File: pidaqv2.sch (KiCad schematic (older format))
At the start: 12 parts, among them J1 Raspberry_Pi_2_3, U1 INA2126E_250

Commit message: ads1261
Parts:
- removed C1, C8, C9: 0.1uF, Capacitor_SMD:C_0805_2012Metric_Pad1.15x1.40mm_HandSolder, symbol Device:C_Small
- removed J1: Raspberry_Pi_2_3, Connector_PinHeader_2.54mm:PinHeader_2x20_P2.54mm_Vertical, symbol Connector:Raspberry_Pi_2_3
- removed JAIN0: Screw_Terminal_01x10, TerminalBlock_TE-Connectivity:TerminalBlock_TE_1-282834-0_1x10_P2.54mm_Horizontal, symbol Connector:Screw_Terminal_01x10
- removed JAIN1: Screw_Terminal_01x12, TerminalBlock_TE-Connectivity:TerminalBlock_TE_1-282834-2_1x12_P2.54mm_Horizontal, symbol Connector:Screw_Terminal_01x12
- removed JLC1, JTC-1: Screw_Terminal_01x06, TerminalBlock_TE-Connectivity:TerminalBlock_TE_282834-6_1x06_P2.54mm_Horizontal, symbol Connector:Screw_Terminal_01x06
- removed MK1, MK2, MK3: MountingHole_Pad, MountingHole:MountingHole_2.7mm_M2.5_ISO14580_Pad, symbol Mechanical:MountingHole_Pad
- removed U1: INA2126E_250, footprints:INA2126E&slash_250, symbol ina2126:INA2126E_250
- added C101, C102: 0.1uF, Capacitor_SMD:C_0603_1608Metric, symbol Device:C
- added H101, H102, H103, H104: MountingHole, MountingHole:MountingHole_3.2mm_M3_ISO7380, symbol Mechanical:MountingHole
- added J101: Conn_02x04_Odd_Even, Connector_PinHeader_2.54mm:PinHeader_2x04_P2.54mm_Vertical, symbol Connector_Generic:Conn_02x04_Odd_Even
- added J102: Conn_01x03, Connector_PinHeader_2.54mm:PinHeader_1x03_P2.54mm_Vertical, symbol Connector_Generic:Conn_01x03
- added J103: Screw_Terminal_01x10, TerminalBlock_Phoenix:TerminalBlock_Phoenix_MKDS-1,5-10-5.08_1x10_P5.08mm_Horizontal, symbol Connector:Screw_Terminal_01x10
- added J104, J106: Screw_Terminal_01x08, TerminalBlock_Phoenix:TerminalBlock_Phoenix_MPT-0,5-8-2.54_1x08_P2.54mm_Horizontal, symbol Connector:Screw_Terminal_01x08
- added J105: Screw_Terminal_01x06, TerminalBlock_Phoenix:TerminalBlock_Phoenix_MKDS-3-6-5.08_1x06_P5.08mm_Horizontal, symbol Connector:Screw_Terminal_01x06
- added J107: Conn_01x01_Female, Connector_PinHeader_2.54mm:PinHeader_1x01_P2.54mm_Vertical, symbol Connector:Conn_01x01_Female
- added U101: INA2126E_250, footprints:INA2126E&slash_250, symbol ins2126:INA2126E_250
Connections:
- net labels added: 2.5V, GNDREF, GPIO, TC-, TC0, TC1, TC2, TC3, TC4, TC5, TC6, TC7, ~CS0, ~CS1
- net labels removed: +2.5V, GNDPWR, ~CE0, ~CE1
- wire segments 70 -> 42
- no-connect marks 4 -> 5
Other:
- note removed: "ID_SD and ID_SC PINS:\nThese pins are reserved for HAT ID EEPROM.\n\nAt boot time this I2C interface will be\ninterrogated to look for an EEPROM\nthat identifes the attached board and\nallows automagic setup of the GPIOs\n(and optionally, Linux drivers).\n\nDO NOT USE these pins for anything other\nthan attaching an I2C ID EEPROM. Leave\nunconnected if ID EEPROM not required."
- note removed: "INA2126 comes with free 5x gain\n"
- note removed: "This ADC is set up for use of the internal PGA (GAINS).\nAll inputs should be in the range of 2.5V +/- 2V\n\nExcel calculator: https://www.ti.com/tool/ADS124S08-EXCEL-CALC-TOOL\n"
- note removed: "Tie negative inputs of thermocouples to +2.5V\n"

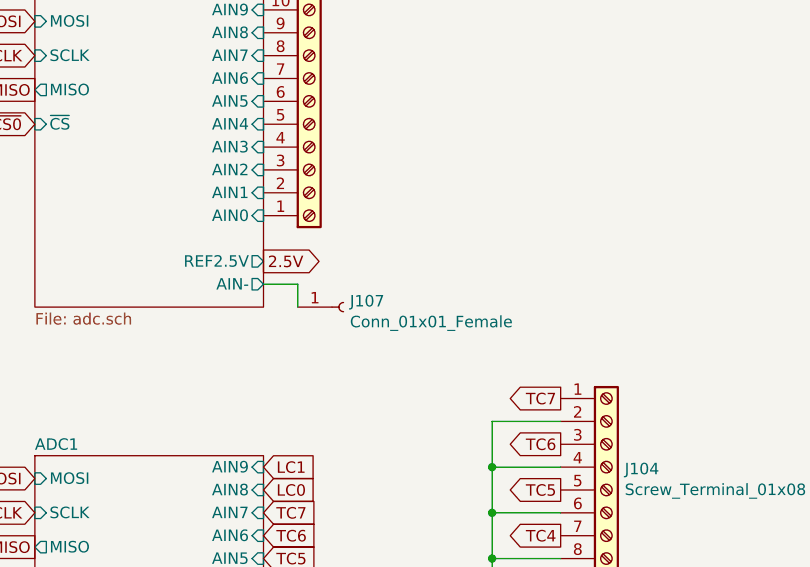
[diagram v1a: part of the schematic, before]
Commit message: last highfreq
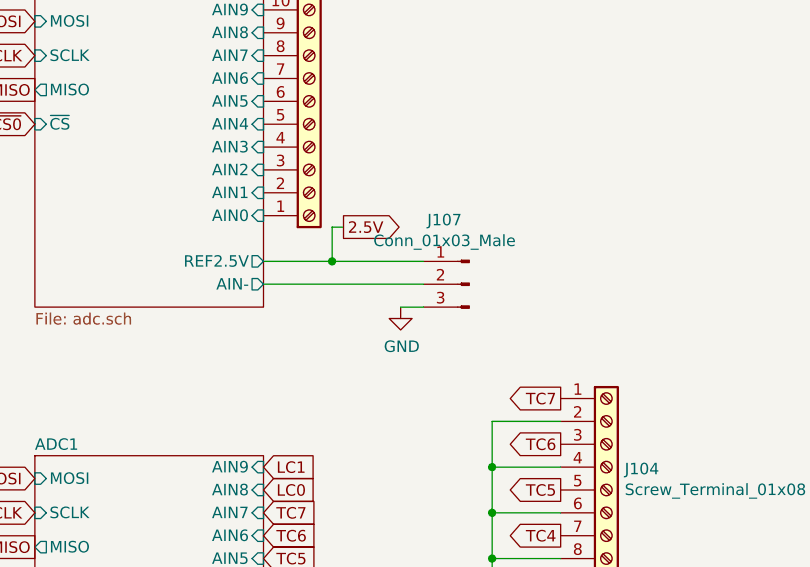
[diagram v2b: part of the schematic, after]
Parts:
- removed J107: Conn_01x01_Female, Connector_PinHeader_2.54mm:PinHeader_1x01_P2.54mm_Vertical, symbol Connector:Conn_01x01_Female
- added J107: Conn_01x03_Male, Connector_PinSocket_2.54mm:PinSocket_1x03_P2.54mm_Vertical, symbol Connector:Conn_01x03_Male
- J101, J102, J103, J104, J105, J106: DNP? (none) -> DNP
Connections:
- net 2.5V: now also J107.1 (Pin_1)
- net ADC0/AIN-: now also J107.2 (Pin_2)
- net GND: now also J107.3 (Pin_3)
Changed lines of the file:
@@
 F 2 "Connector_PinHeader_2.54mm:PinHeader_2x04_P2.54mm_Vertical" H 1400 1950 50  0001 C CNN
 F 3 "~" H 1400 1950 50  0001 C CNN
+F 4 "DNP" H 1400 1950 50  0001 C CNN "DNP?"
 	1    1400 1950
 	-1   0    0    -1
@@
 F 2 "TerminalBlock_Phoenix:TerminalBlock_Phoenix_MKDS-1,5-10-5.08_1x10_P5.08mm_Horizontal" H 2100 4050 50  0001 C CNN
 F 3 "~" H 2100 4050 50  0001 C CNN
+F 4 "DNP" H 2100 4050 50  0001 C CNN "DNP?"
 	1    2100 4050
 	1    0    0    1
@@
 F 2 "TerminalBlock_Phoenix:TerminalBlock_Phoenix_MKDS-3-6-5.08_1x06_P5.08mm_Horizontal" H 8350 5450 50  0001 C CNN
 F 3 "~" H 8350 5450 50  0001 C CNN
+F 4 "DNP" H 8350 5450 50  0001 C CNN "DNP?"
 	1    8350 5450
 	1    0    0    -1
@@
 	1    0    0    -1
 $EndComp
-Text GLabel 1900 4650 2    50   Output ~ 0
+Text GLabel 2250 4500 2    50   Output ~ 0
 2.5V
 Text GLabel 1900 6750 2    50   Output ~ 0
@@
 F 2 "TerminalBlock_Phoenix:TerminalBlock_Phoenix_MPT-0,5-8-2.54_1x08_P2.54mm_Horizontal" H 3400 5550 50  0001 C CNN
 F 3 "~" H 3400 5550 50  0001 C CNN
+F 4 "DNP" H 3400 5550 50  0001 C CNN "DNP?"
 	1    3400 5550
 	1    0    0    -1
@@
 F 2 "TerminalBlock_Phoenix:TerminalBlock_Phoenix_MPT-0,5-8-2.54_1x08_P2.54mm_Horizontal" H 3400 6550 50  0001 C CNN
 F 3 "~" H 3400 6550 50  0001 C CNN
+F 4 "DNP" H 3400 6550 50  0001 C CNN "DNP?"
 	1    3400 6550
 	1    0    0    -1
@@
 F 2 "Connector_PinHeader_2.54mm:PinHeader_1x03_P2.54mm_Vertical" H 1450 1200 50  0001 C CNN
 F 3 "~" H 1450 1200 50  0001 C CNN
+F 4 "DNP" H 1450 1200 50  0001 C CNN "DNP?"
 	1    1450 1200
 	1    0    0    -1
@@
 $EndComp
 $Comp
-L Connector:Conn_01x01_Female J107
-U 1 1 5F4B9AB1
-P 2250 4850
-F 0 "J107" H 2278 4876 50  0000 L CNN
-F 1 "Conn_01x01_Female" H 2278 4785 50  0000 L CNN
-F 2 "Connector_PinHeader_2.54mm:PinHeader_1x01_P2.54mm_Vertical" H 2250 4850 50  0001 C CNN
-F 3 "~" H 2250 4850 50  0001 C CNN
-	1    2250 4850
-	1    0    0    -1
-$EndComp
-Wire Wire Line
-	1900 4750 2050 4750
-Wire Wire Line
-	2050 4750 2050 4850
+L Connector:Conn_01x03_Male J107
+U 1 1 5F5328B6
+P 2800 4750
+F 0 "J107" H 2908 5031 50  0000 C CNN
+F 1 "Conn_01x03_Male" H 2908 4940 50  0000 C CNN
+F 2 "Connector_PinSocket_2.54mm:PinSocket_1x03_P2.54mm_Vertical" H 2800 4750 50  0001 C CNN
+F 3 "~" H 2800 4750 50  0001 C CNN
+	1    2800 4750
+	-1   0    0    -1
+$EndComp
+$Comp
+L power:GND #PWR0114
+U 1 1 5F539769
+P 2500 4850
+F 0 "#PWR0114" H 2500 4600 50  0001 C CNN
+F 1 "GND" H 2505 4677 50  0000 C CNN
+F 2 "" H 2500 4850 50  0001 C CNN
+F 3 "" H 2500 4850 50  0001 C CNN
+	1    2500 4850
+	1    0    0    -1
+$EndComp
+Wire Wire Line
+	2500 4850 2600 4850
+Wire Wire Line
+	1900 4650 2200 4650
+Wire Wire Line
+	2250 4500 2200 4500
+Wire Wire Line
+	2200 4500 2200 4650
+Connection ~ 2200 4650
+Wire Wire Line
+	2200 4650 2600 4650
+Wire Wire Line
+	1900 4750 2600 4750
 $EndSCHEMATC

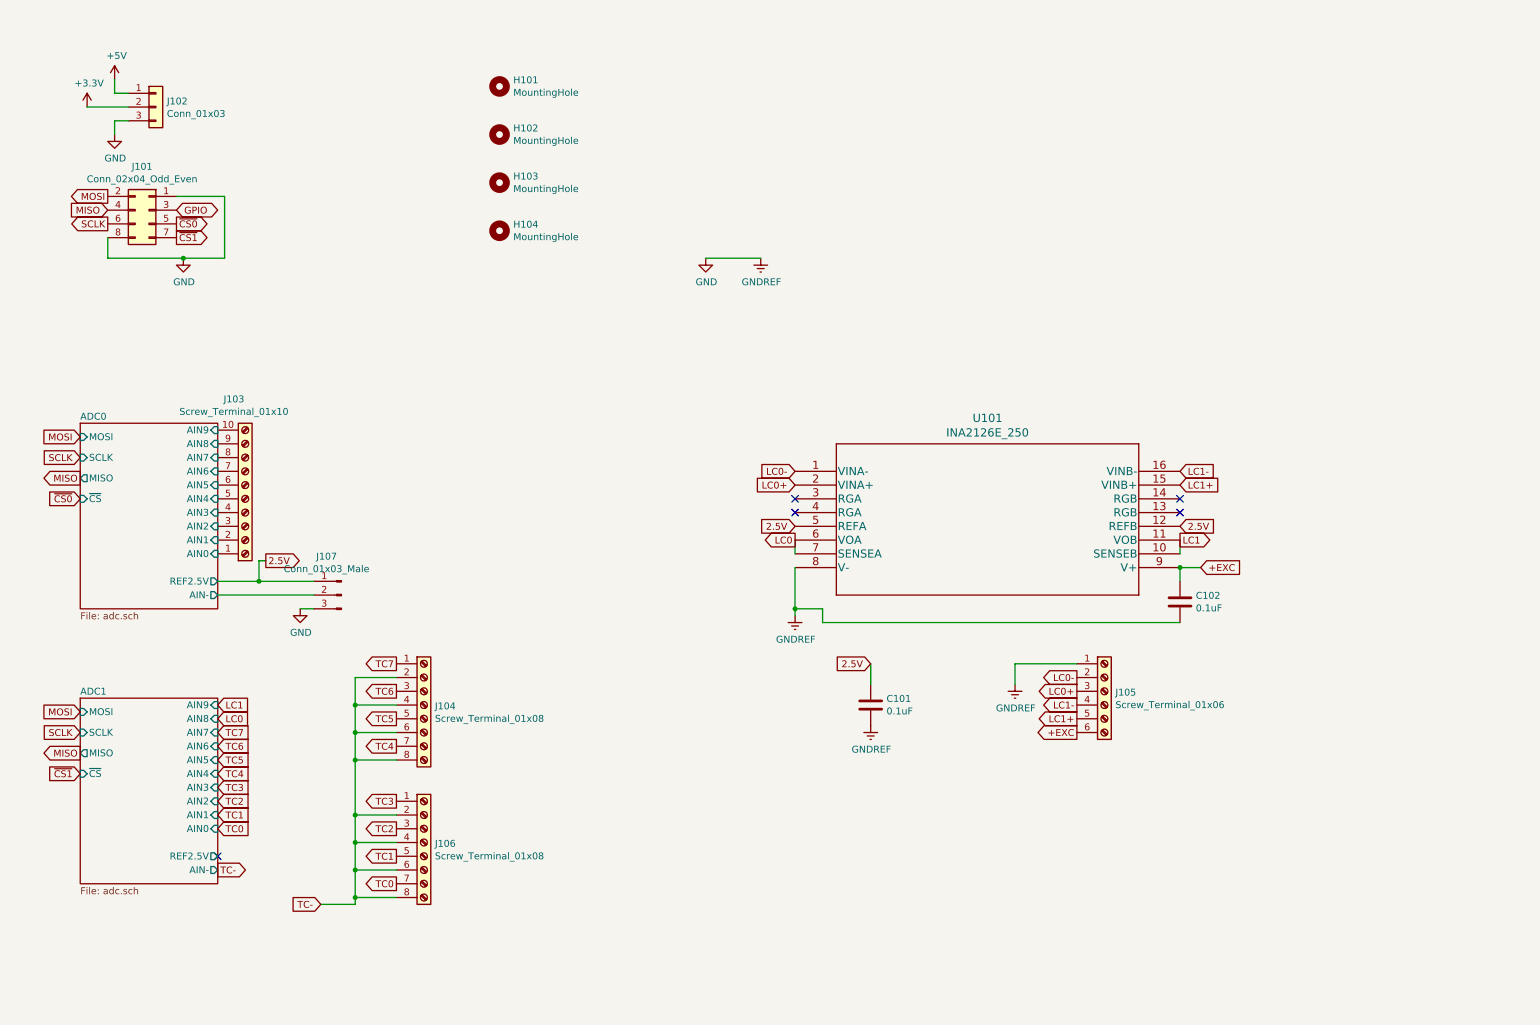
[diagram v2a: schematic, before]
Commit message: boi did i cut up that ground plane
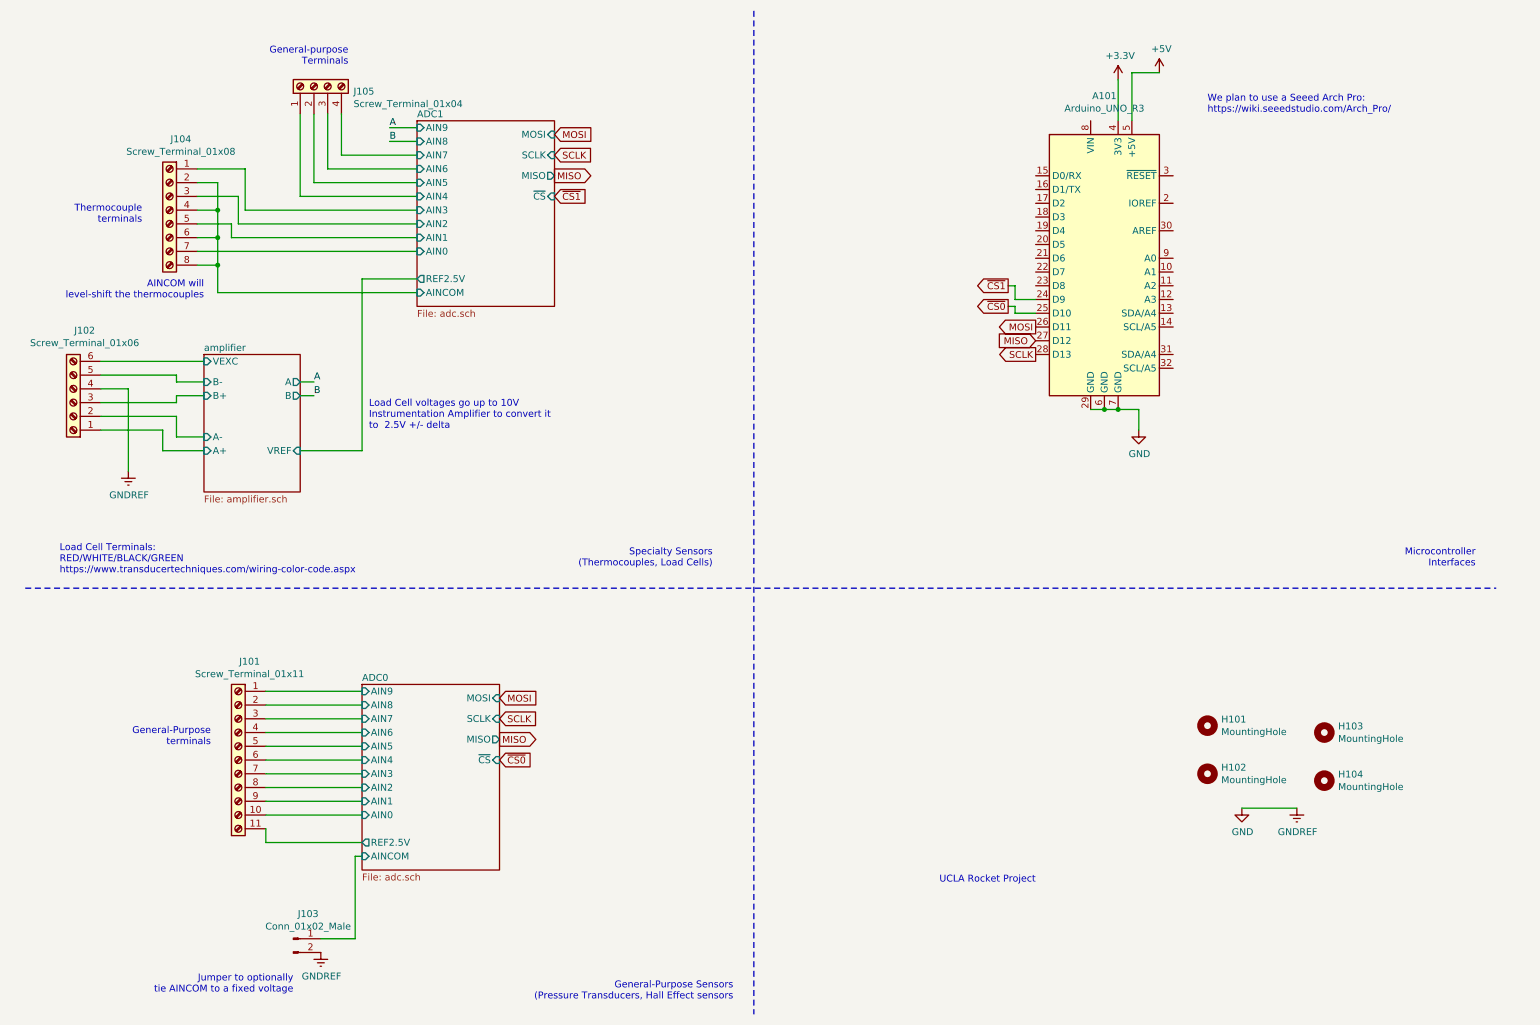
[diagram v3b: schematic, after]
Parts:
- removed C101, C102: 0.1uF, Capacitor_SMD:C_0603_1608Metric, symbol Device:C
- removed J101: Conn_02x04_Odd_Even, Connector_PinHeader_2.54mm:PinHeader_2x04_P2.54mm_Vertical, symbol Connector_Generic:Conn_02x04_Odd_Even
- removed J102: Conn_01x03, Connector_PinHeader_2.54mm:PinHeader_1x03_P2.54mm_Vertical, symbol Connector_Generic:Conn_01x03
- removed J103: Screw_Terminal_01x10, TerminalBlock_Phoenix:TerminalBlock_Phoenix_MKDS-1,5-10-5.08_1x10_P5.08mm_Horizontal, symbol Connector:Screw_Terminal_01x10
- removed J105: Screw_Terminal_01x06, TerminalBlock_Phoenix:TerminalBlock_Phoenix_MKDS-3-6-5.08_1x06_P5.08mm_Horizontal, symbol Connector:Screw_Terminal_01x06
- removed J106: Screw_Terminal_01x08, TerminalBlock_Phoenix:TerminalBlock_Phoenix_MPT-0,5-8-2.54_1x08_P2.54mm_Horizontal, symbol Connector:Screw_Terminal_01x08
- removed J107: Conn_01x03_Male, Connector_PinSocket_2.54mm:PinSocket_1x03_P2.54mm_Vertical, symbol Connector:Conn_01x03_Male
- removed U101: INA2126E_250, footprints:INA2126E&slash_250, symbol ins2126:INA2126E_250
- added A101: Arduino_UNO_R3, Module:Arduino_UNO_R3, symbol MCU_Module:Arduino_UNO_R3
- added J101: Screw_Terminal_01x11, TerminalBlock_Phoenix:TerminalBlock_Phoenix_MKDS-3-11-5.08_1x11_P5.08mm_Horizontal, symbol Connector:Screw_Terminal_01x11
- added J102: Screw_Terminal_01x06, TerminalBlock_Phoenix:TerminalBlock_Phoenix_MKDS-1,5-6-5.08_1x06_P5.08mm_Horizontal, symbol Connector:Screw_Terminal_01x06
- added J103: Conn_01x02_Male, Connector_PinHeader_2.54mm:PinHeader_1x02_P2.54mm_Vertical, symbol Connector:Conn_01x02_Male
- added J105: Screw_Terminal_01x04, TerminalBlock_Phoenix:TerminalBlock_Phoenix_MPT-0,5-4-2.54_1x04_P2.54mm_Horizontal, symbol Connector:Screw_Terminal_01x04
- J104: DNP? DNP -> (none)
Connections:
- net +3V3: now also A101.4 (3V3)
- net +5V: now also A101.5 (+5V)
- net ADC0/AIN0: now also J101.10 (Pin_10)
- net ADC0/AIN1: now also J101.9 (Pin_9)
- net ADC0/AIN2: now also J101.8 (Pin_8)
- net ADC0/AIN3: now also J101.7 (Pin_7)
- net ADC0/AIN4: now also J101.6 (Pin_6)
- net ADC0/AIN5: now also J101.5 (Pin_5)
- net ADC0/AIN6: now also J101.4 (Pin_4)
- net ADC0/AIN7: now also J101.3 (Pin_3)
- net ADC0/AIN8: now also J101.2 (Pin_2)
- net ADC0/AIN9: now also J101.1 (Pin_1)
- net GND: now also A101.29 (GND), A101.6 (GND), A101.7 (GND), J102.4 (Pin_4), J103.2 (Pin_2)
- net MISO: now also A101.27 (D12)
- net MOSI: now also A101.26 (D11)
- net SCLK: now also A101.28 (D13)
- net ~CS0: now also A101.25 (D10)
- net ~CS1: now also A101.24 (D9)
- net TC- renamed ADC1/AINCOM
- net TC4 renamed ADC1/AIN0
- net TC5 renamed ADC1/AIN1
- net TC6 renamed ADC1/AIN2
- net TC7 renamed ADC1/AIN3
- new net ADC0/AINCOM: J103.1 (Pin_1)
- new net ADC0/REF2.5V: J101.11 (Pin_11)
- new net ADC1/AIN4: J105.1 (Pin_1)
- new net ADC1/AIN5: J105.2 (Pin_2)
- new net ADC1/AIN6: J105.3 (Pin_3)
- new net ADC1/AIN7: J105.4 (Pin_4)
- new net amplifier/A+: J102.1 (Pin_1)
- new net amplifier/A-: J102.2 (Pin_2)
- new net amplifier/B+: J102.3 (Pin_3)
- new net amplifier/B-: J102.5 (Pin_5)
- new net amplifier/VEXC: J102.6 (Pin_6)
- no-connect marks 5 -> 0
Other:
- note added: "AINCOM will \nlevel-shift the thermocouples\n"
- note added: "General-Purpose Sensors\n(Pressure Transducers, Hall Effect sensors"
- note added: "General-Purpose\nterminals"
- note added: "General-purpose\nTerminals"
- note added: "Jumper to optionally\ntie AINCOM to a fixed voltage"
- note added: "Load Cell Terminals:\nRED/WHITE/BLACK/GREEN\nhttps://www.transducertechniques.com/wiring-color-code.aspx"
- note added: "Load Cell voltages go up to 10V\nInstrumentation Amplifier to convert it\nto 2.5V +/- delta"
- note added: "Microcontroller\nInterfaces"
- note added: "Specialty Sensors\n(Thermocouples, Load Cells)"
- note added: "Thermocouple\nterminals"
- note added: "UCLA Rocket Project"
- note added: "We plan to use a Seeed Arch Pro:\nhttps://wiki.seeedstudio.com/Arch_Pro/"
- moved on the sheet: H101, H102, H103, H104
